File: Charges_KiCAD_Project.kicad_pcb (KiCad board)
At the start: 4 copper layers, 79.2 x 87.2 mm, 43 parts, among them IC1 TP124005-2, IC2 STM32L562VET6Q, J1 TB002-500-04BE, J2 TB002-500-04BE, J3 L717SDC37P1ACH4F, Q1 SI7232DN-T1-GE3, Q2 SI7232DN-T1-GE3, U1 MS5607-02BA

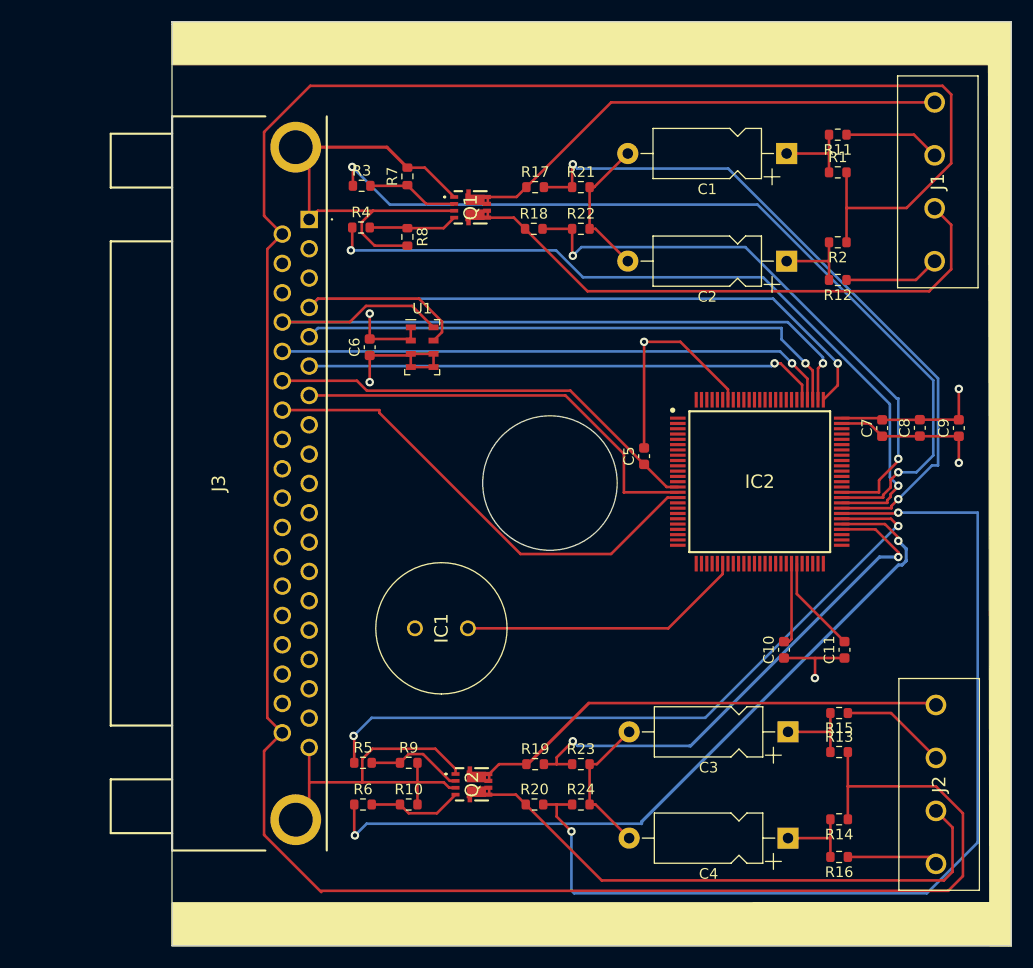
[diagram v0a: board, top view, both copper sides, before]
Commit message: updated board
updated the board again
added a crystal
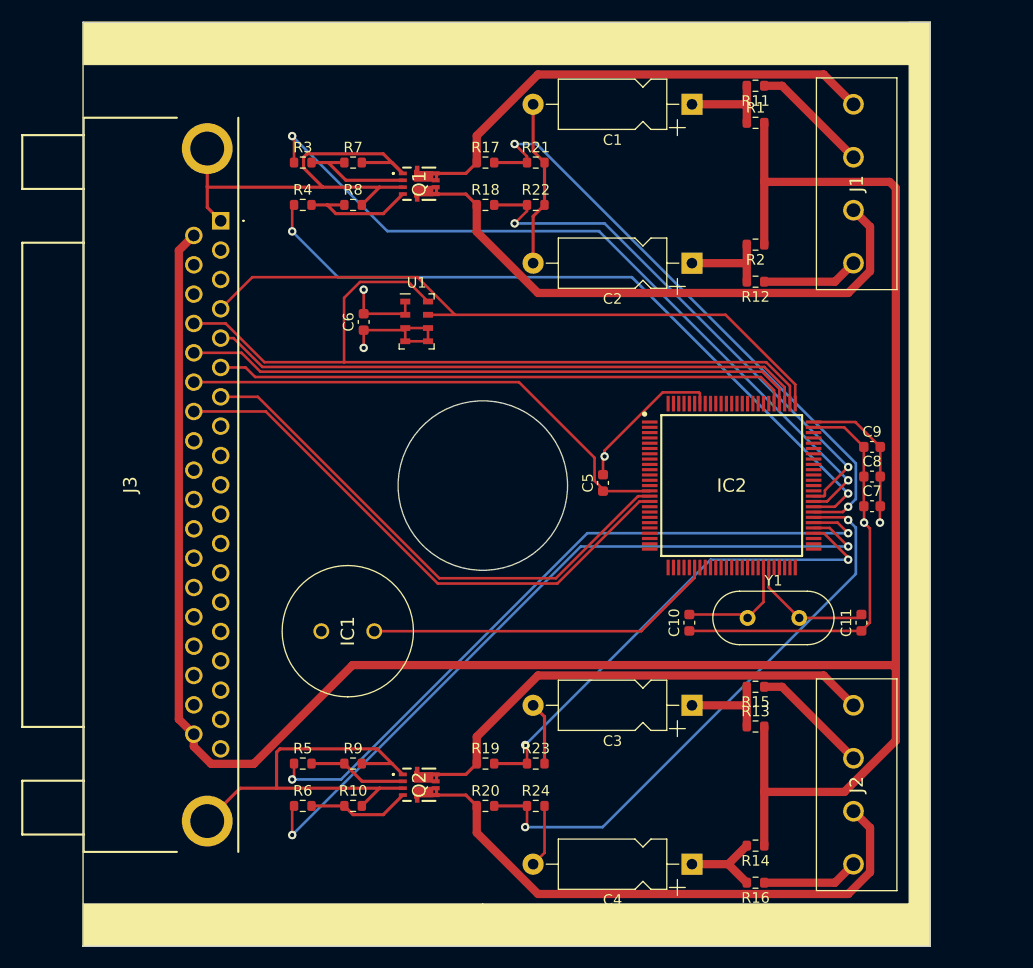
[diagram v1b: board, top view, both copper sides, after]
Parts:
- added Y1: 32mhz, Crystal:Crystal_HC49-4H_Vertical, F.Cu at (151.2, 108.8)
- moved C1 10.1 mm to (146.0, 60.2)
- moved C3 9.41 mm to (146.0, 117.0)
- moved C4 9.39 mm to (146.0, 132.0)
- moved C10 9.30 mm to (145.8, 109.2)
- moved R1 9.06 mm to (152.0, 62.0)
- moved R11 9.04 mm to (152.0, 58.5)
- moved C2 8.94 mm to (146.0, 75.2)
- moved IC1 8.85 mm to (116.0, 110.0)
- moved C9 8.39 mm to (163.0, 92.6), turned to 0 degrees
- moved J3 8.36 mm to (101.5, 71.2)
- moved R14 8.28 mm to (152.0, 130.2)
- moved R15 8.27 mm to (152.0, 115.2)
- moved R16 8.26 mm to (152.0, 133.8)
- moved R13 8.25 mm to (152.0, 119.0)
- moved J2 7.79 mm to (161.2, 117.0)
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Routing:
- net /Sense_D: track 96.0 -> 55.1 mm
- net +5V: track 253.7 -> 222.4 mm
- net GND: track 168.9 -> 182.4 mm, vias 4 -> 3
- net /Fire_A: track 83.0 -> 72.6 mm
- net /Fire: track 40.7 -> 50.8 mm
- net /Sense_A: track 66.8 -> 57.9 mm
- net /SWDIO: track 72.7 -> 64.0 mm, vias 1 -> 0
- net /Fire_Redundant: track 45.3 -> 53.0 mm
- net /NRST: track 41.5 -> 48.7 mm
- net /Buzzer_Excitation: track 27.2 -> 33.3 mm
- net /Alert_sda: track 52.6 -> 58.1 mm, vias 1 -> 0
- net /Alert_Active: track 49.6 -> 54.4 mm, vias 1 -> 0
- net /Fire_B: track 73.7 -> 69.1 mm
- net /Sense_B: track 55.5 -> 51.0 mm
- net /Alert_scl: track 52.9 -> 56.7 mm, vias 1 -> 0
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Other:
- board size 79.2 x 87.2 mm -> 80 x 87.2 mm
